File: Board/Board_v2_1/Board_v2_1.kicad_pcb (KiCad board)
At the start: 2 copper layers, 83.5 x 75 mm, 22 parts, among them M1 MountingHole_2.2mm_M2_ISO7380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, M2 MountingHole_2.2mm_M2_ISO7380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, M3 MountingHole_2.2mm_M2_ISO7380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, M4 MountingHole_2.2mm_M2_ISO7380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

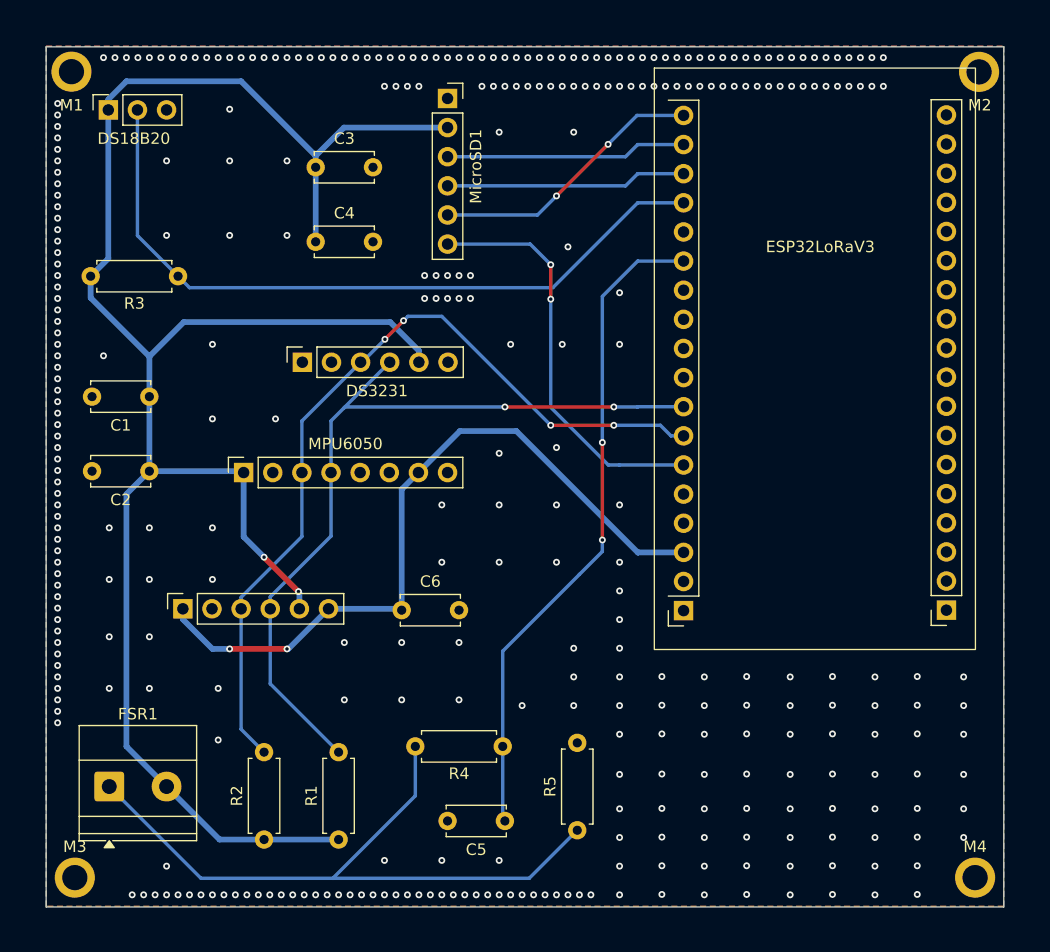
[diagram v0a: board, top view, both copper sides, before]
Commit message: Versión final de pcb
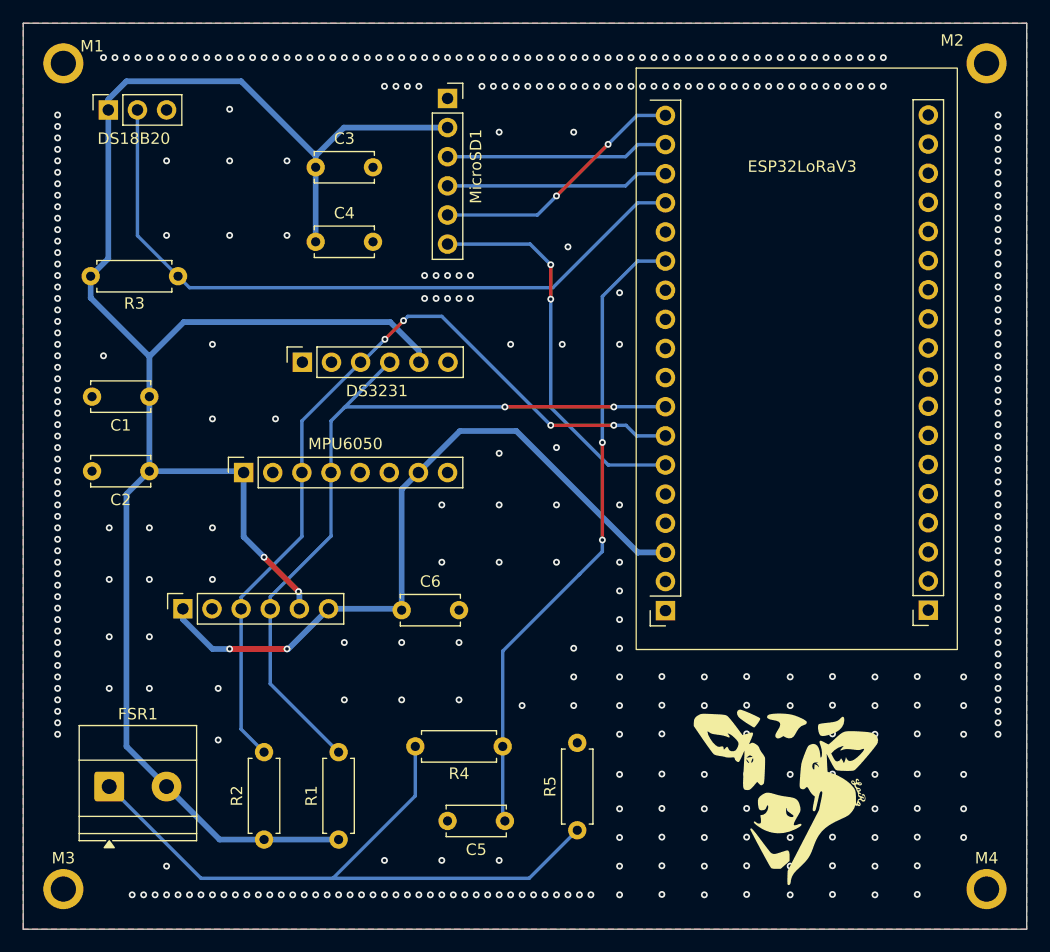
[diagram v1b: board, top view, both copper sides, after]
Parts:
- added G***: LOGO, Battery:vaca2, F.Cu at (84.0, 84.0)
- moved ESP32LoRaV3 1.58 mm to (85.0, 46.4)
- moved M3 1.41 mm to (21.0, 92.0)
- moved M4 1.41 mm to (101.5, 92.0)
- moved M1 1.01 mm to (21.0, 20.0)
- moved M2 0.99 mm to (101.5, 20.0)
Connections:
- M1 pad 1: (no net) -> GND
- M2 pad 2: (no net) -> GND
- M4 pad 4: (no net) -> GND
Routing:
- net /MISO: track 21.0 -> 19.4 mm
- net /TEMP: track 63.5 -> 61.9 mm
- net /SDA: track 70.4 -> 68.8 mm
- net /SCK: track 24.2 -> 22.7 mm
- net /CS: track 35.8 -> 34.3 mm
- net /MOSI: track 21.0 -> 19.4 mm
- net /FSR: track 57.8 -> 56.2 mm
- net +3V3: track 64.2 -> 62.6 mm
- net /SCL: track 73.3 -> 71.7 mm
- net GND: vias 342 -> 397
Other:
- board size 83.5 x 75 mm -> 87.5 x 79 mm
